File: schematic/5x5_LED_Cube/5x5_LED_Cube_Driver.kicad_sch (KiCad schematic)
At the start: 19 parts, among them J1 Power, J2 Adafruit_Micro_SD_Card_SPI_SD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, J3 Layers, Q1 DMG2305UX, Q2 DMG2305UX, Q3 DMG2305UX, Q4 DMG2305UX, Q5 DMG2305UX, U1 TLC5940NT, U2 TLC5940NT, U3 Pico

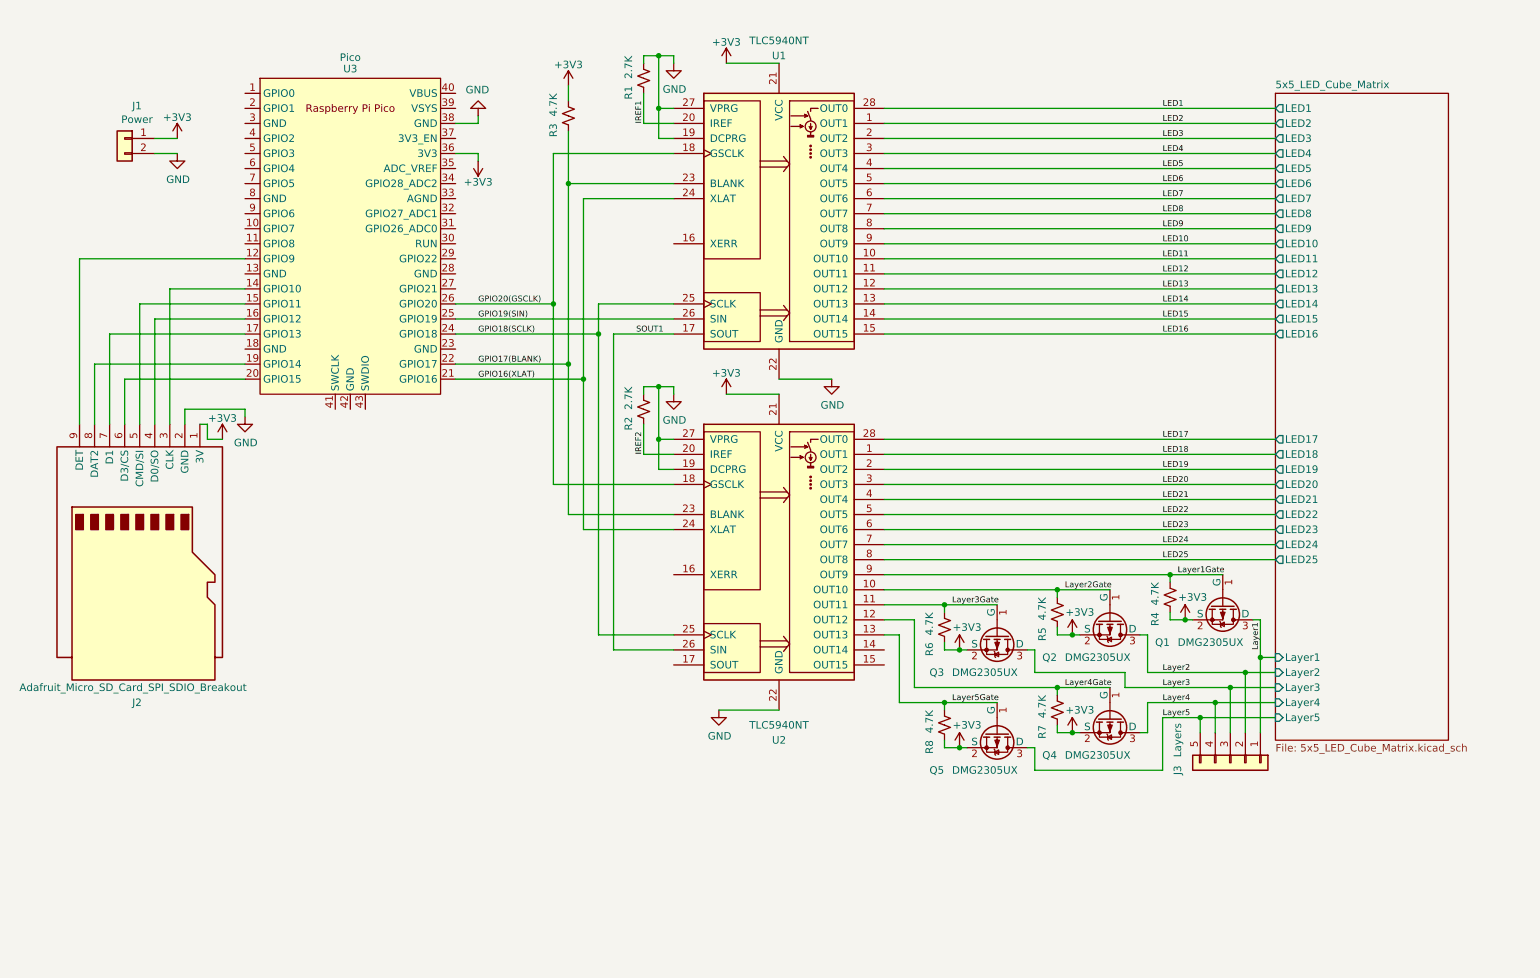
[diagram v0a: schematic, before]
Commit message: Updated schematic and footprints
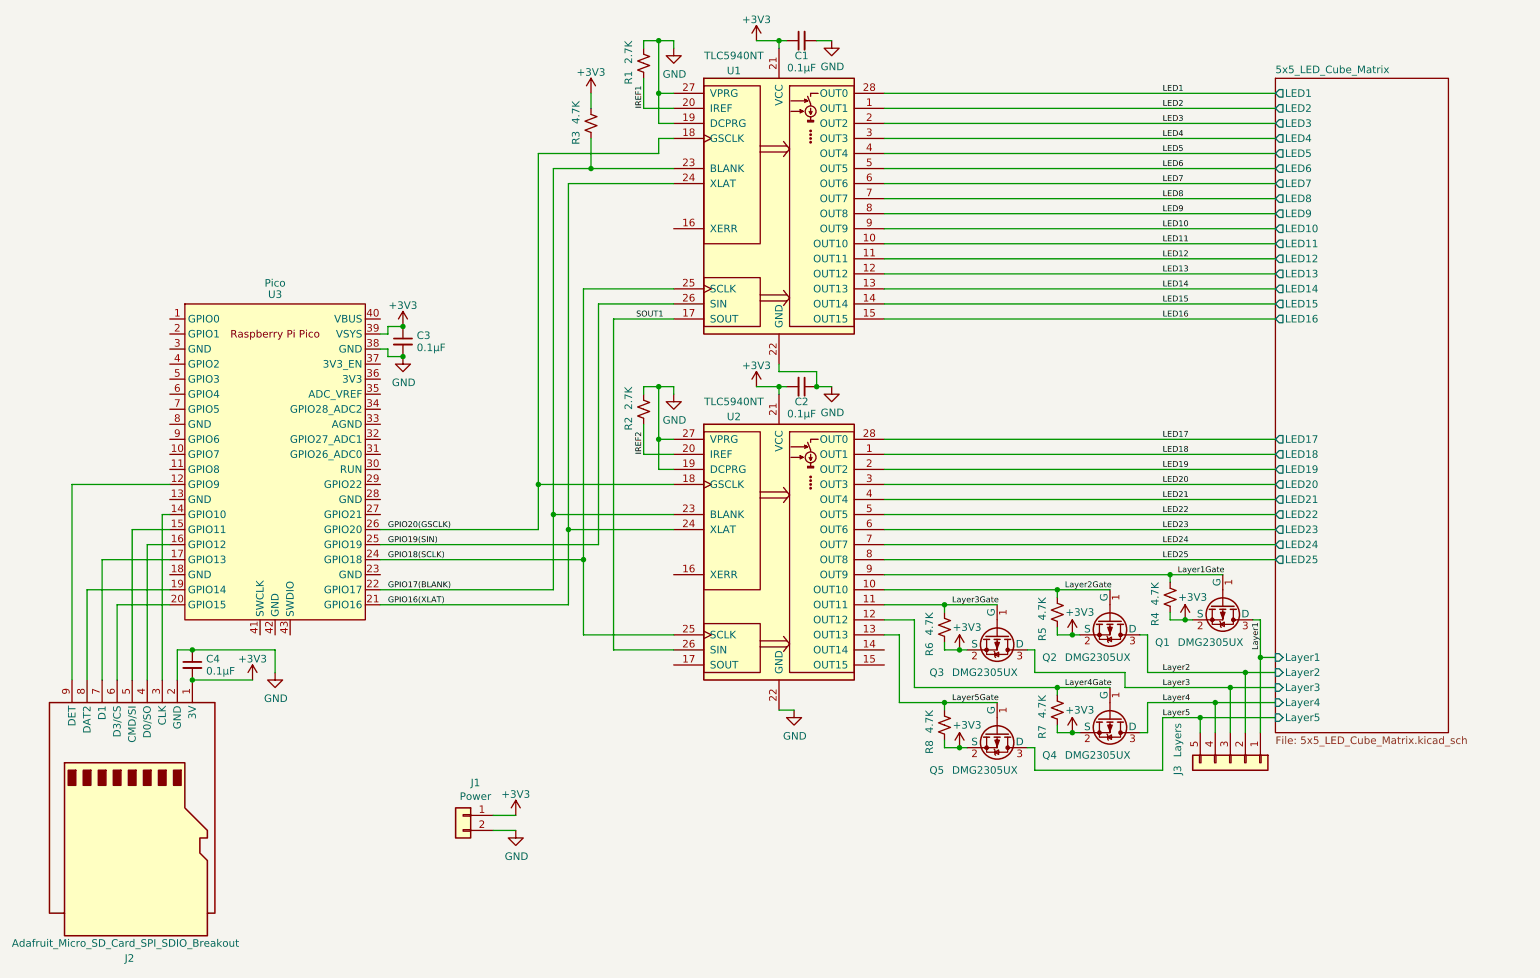
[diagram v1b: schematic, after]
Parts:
- added C1, C2, C3, C4: 0.1µF, Capacitor_SMD:C_0402_1005Metric_Pad0.74x0.62mm_HandSolder, symbol Device:C_Small
- J1: footprint Connector_PinHeader_2.00mm:PinHeader_1x02_P2.00mm_Vertical -> Connector_PinSocket_2.54mm:PinSocket_1x02_P2.54mm_Vertical
- J2: footprint Connector_PinHeader_2.00mm:PinHeader_1x09_P2.00mm_Vertical -> My_Library:Adafruit_Micro_SD_Card_SPI_SDIO_Breakout
- J3: footprint Connector_PinHeader_2.00mm:PinHeader_1x05_P2.00mm_Vertical -> Connector_PinSocket_2.54mm:PinSocket_1x05_P2.54mm_Vertical
- U3: footprint RPi_Pico:RPi_Pico_SMD_TH -> MCU_RaspberryPi_and_Boards:RPi_Pico_SMD_TH
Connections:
- net +3V3: now also U3.39 (VSYS), C1.1, C2.2, C3.1, C4.2; no longer U3.36 (3V3)
- net GND: now also C1.2, C2.1, C3.2, C4.1
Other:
- moved on the sheet: J1, J2, R1, R3, U1, U3
